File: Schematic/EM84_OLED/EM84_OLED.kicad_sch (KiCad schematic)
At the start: 21 parts, among them J1 FFC6, J2 Pin header, U1 ATMEGA328P-AU, U2 MCP6001T-I/OT, U3 Display_OLED_0.91_I2C, U4 NCP1117-5.0_SOT223, Y1 16MHz 16pF

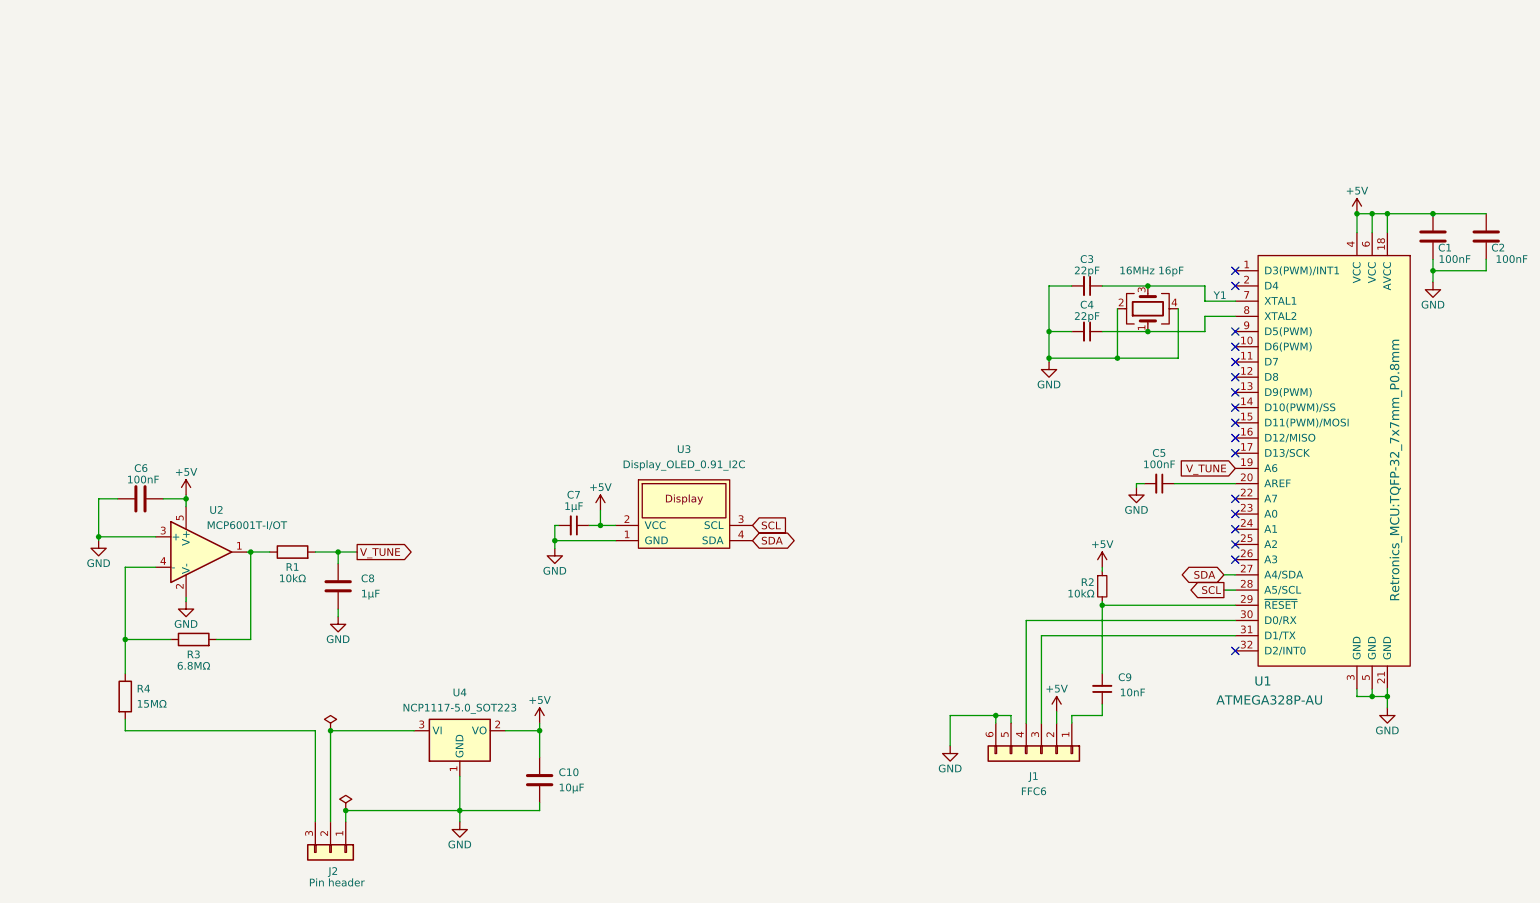
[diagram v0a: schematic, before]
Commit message: File cleanup
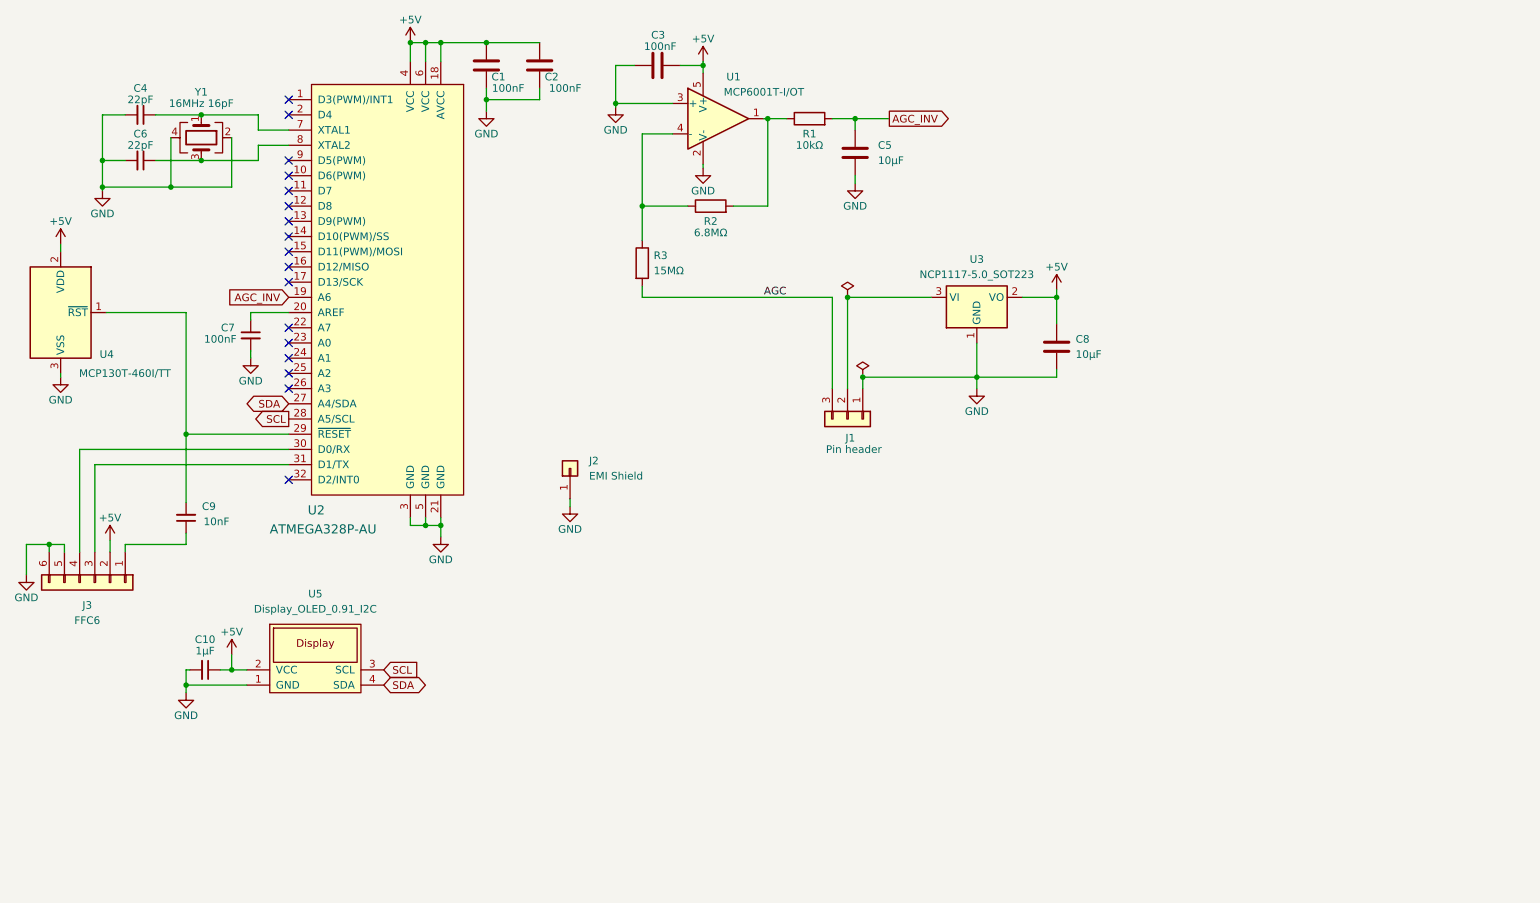
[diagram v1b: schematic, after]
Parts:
- removed R2: 10kΩ, Retronics_Passives:R_0603_1608Metric_Pad0.98x0.95mm_HandSolder, symbol Device:R_Small
- added J2: EMI Shield, Retronics_Hardware:EMI_Shield_MS192-10S, symbol Connector_Generic:Conn_01x01
- added U4: MCP130T-460I/TT, Package_TO_SOT_SMD:SOT-23, symbol Power_Supervisor:MCP130-xxxxTT
- C5: renamed from C8; value 1µF -> 10µF
- J1: renamed from J2; footprint Retronics_Connectors:PinHeader_1x03_P2.54mm_Horizontal -> Retronics_Connectors:PinHeader_1x03_P2.54mm_Horizontal_Alt
- renumbered C7 to C10, C6 to C3, C3 to C4, C4 to C6, C5 to C7, C10 to C8, J1 to J3, R3 to R2, R4 to R3, U2 to U1, U1 to U2, U4 to U3, U3 to U5
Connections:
- net +5V: now also U4.2 (VDD)
- net GND: now also J2.1 (Pin_1), U4.3 (VSS)
- net at C6.1, U2.8 (XTAL2): now also Y1.3; no longer Y1.1
- net at C4.1, U2.7 (XTAL1): now also Y1.1; no longer Y1.3
- net AGC: now reaches J1.3 (Pin_3), R3.2
- net at C9.2, U2.29 (~{RESET}): now also U4.1 (~{RST})
- net V_TUNE renamed AGC_INV
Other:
- moved on the sheet: C1, C10, C2, C3, C4, C5, C6, C7, C8, C9, J1, J3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
